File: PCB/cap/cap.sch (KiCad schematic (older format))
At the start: 24 parts, among them J1 Servo1, J3 LS1, J4 LS2, J5 VCC/GND-IN, J7 FSR1, U1 ACS723xLCTR-05AB, U2 NRF24L01_Breakout, U3 INA181A3

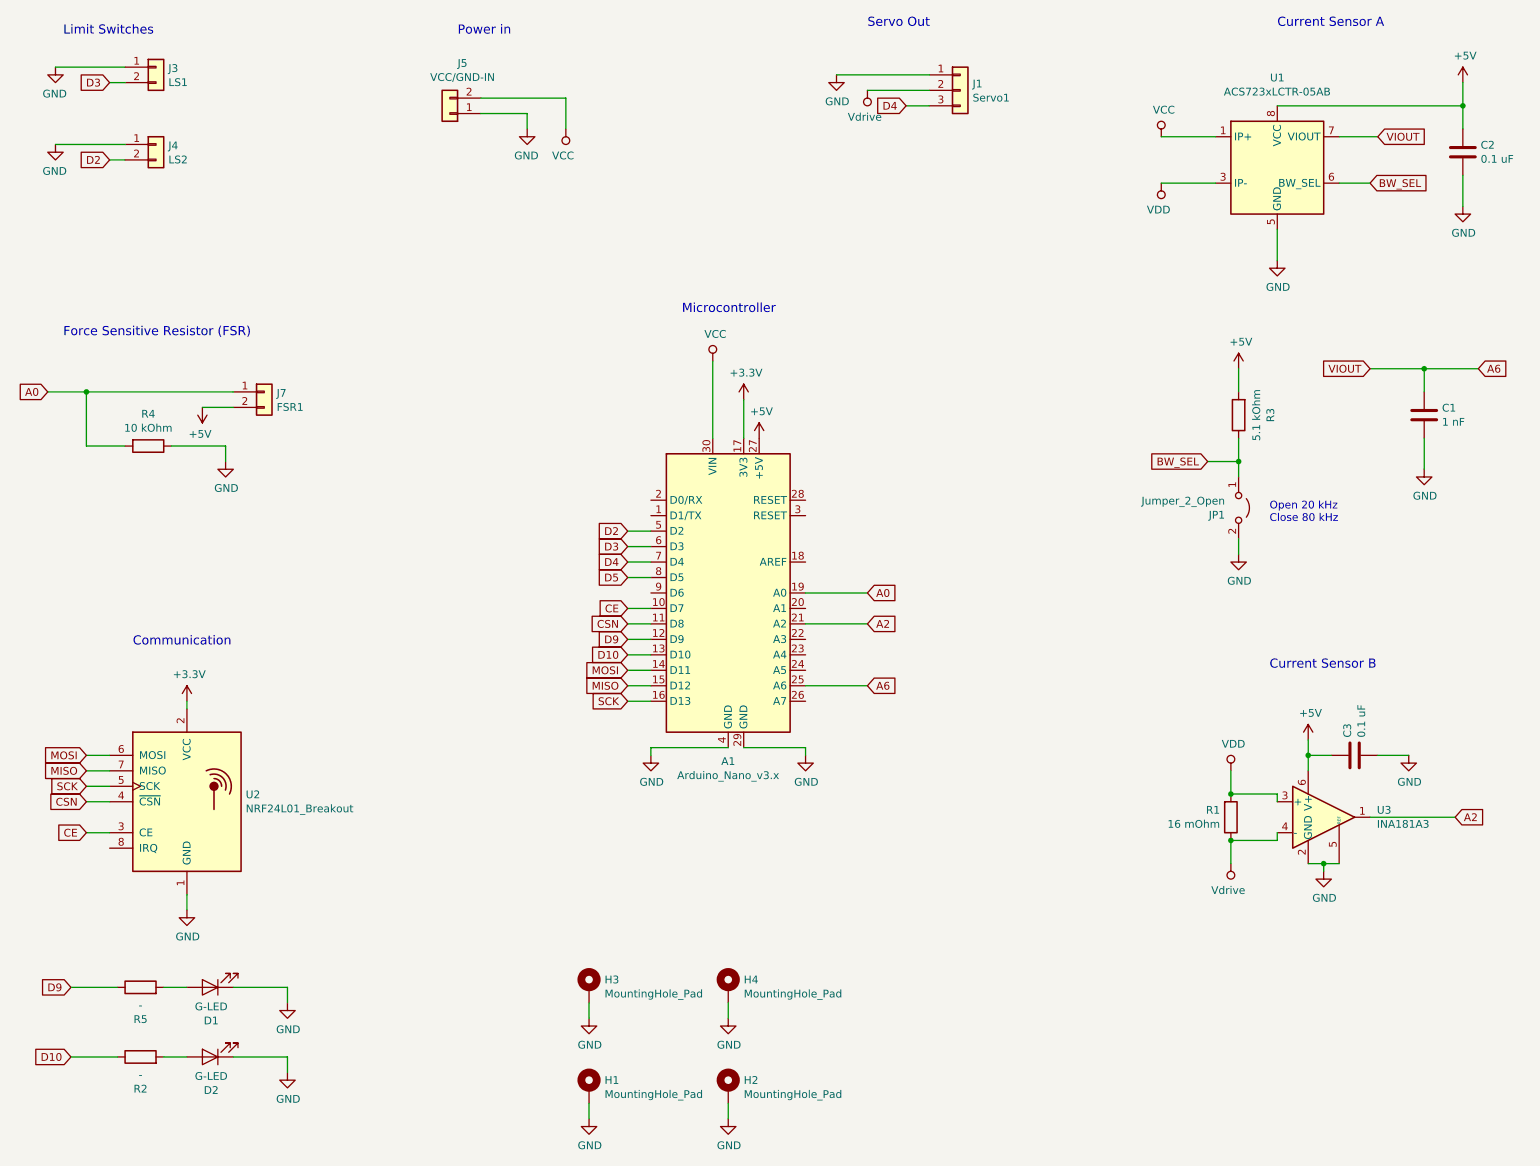
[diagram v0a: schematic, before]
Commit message: All schematics detail check complete
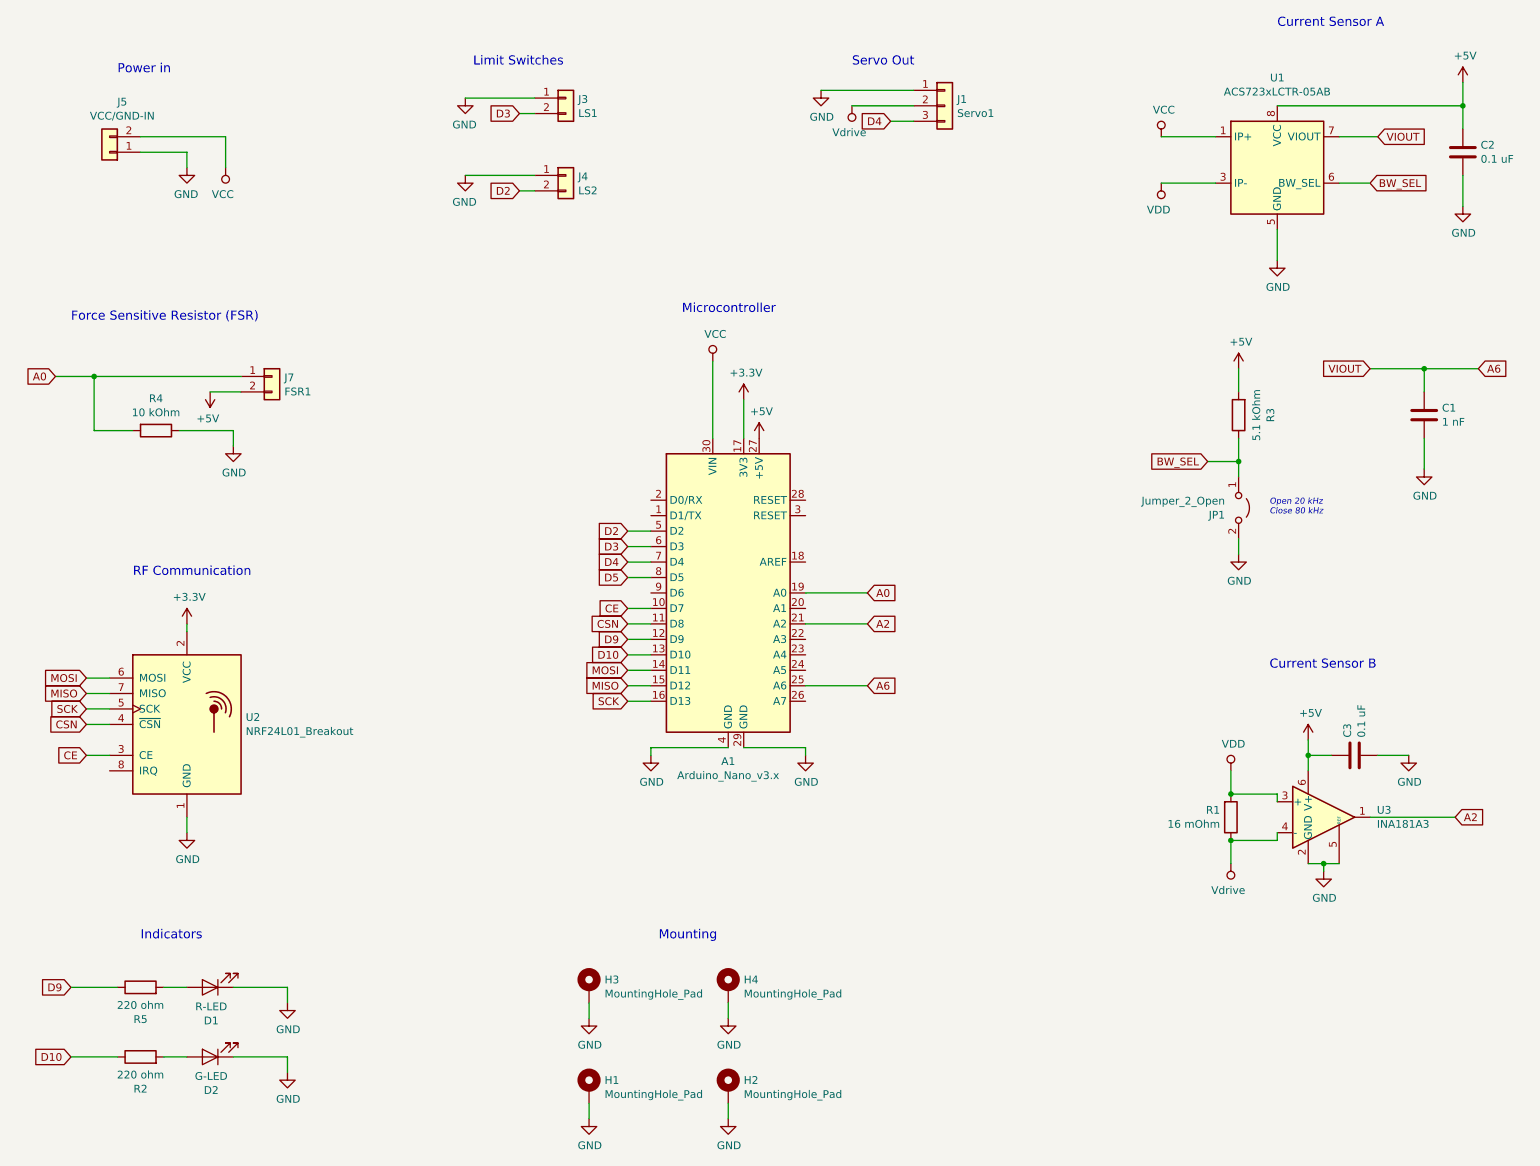
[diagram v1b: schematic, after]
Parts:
- C2, C3: Field4 (none) -> 399-7845-1-ND
- D1: value G-LED -> R-LED; Field4 (none) -> 160-1447-1-ND
- D2: Field4 (none) -> 160-1443-6-ND
- R2, R5: value - -> 220 ohm; Field4 (none) -> P220BZCT-ND
- R4: Field4 (none) -> P10.0KHCT-ND
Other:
- note added: "Indicators"
- note added: "Mounting"
- note added: "RF Communication"
- note removed: "Communication"
- moved on the sheet: J1, J3, J4, J5, J7, R4, U2
